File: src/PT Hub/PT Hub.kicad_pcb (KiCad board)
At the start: 2 copper layers, 18 parts, among them P1 20021511-00026T4LF, P2 39299043, P3 39299043, P4 39299043, P5 39299043, P6 39299043, P7 39299043, P8 39299043, P9 39299043

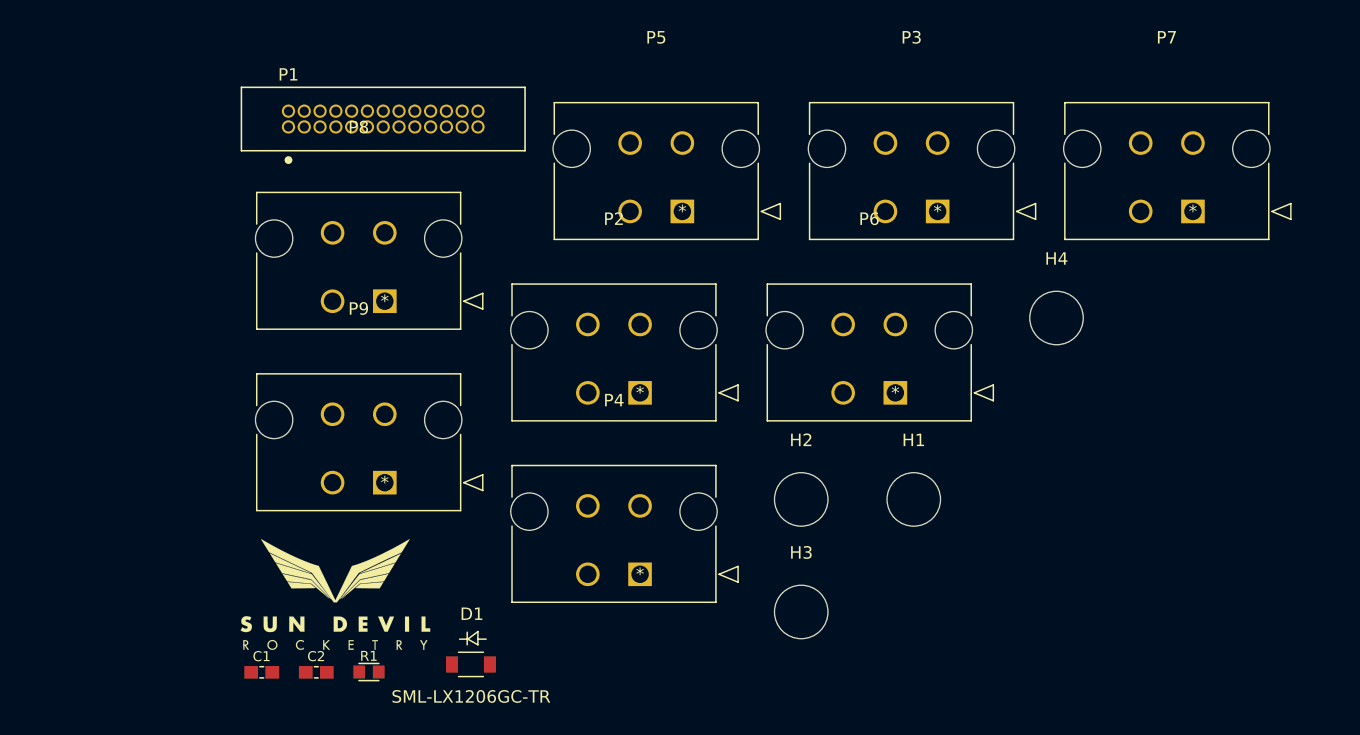
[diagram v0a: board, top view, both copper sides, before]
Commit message: most recent PCB changes as of 7/1
PT Hub PCB changes
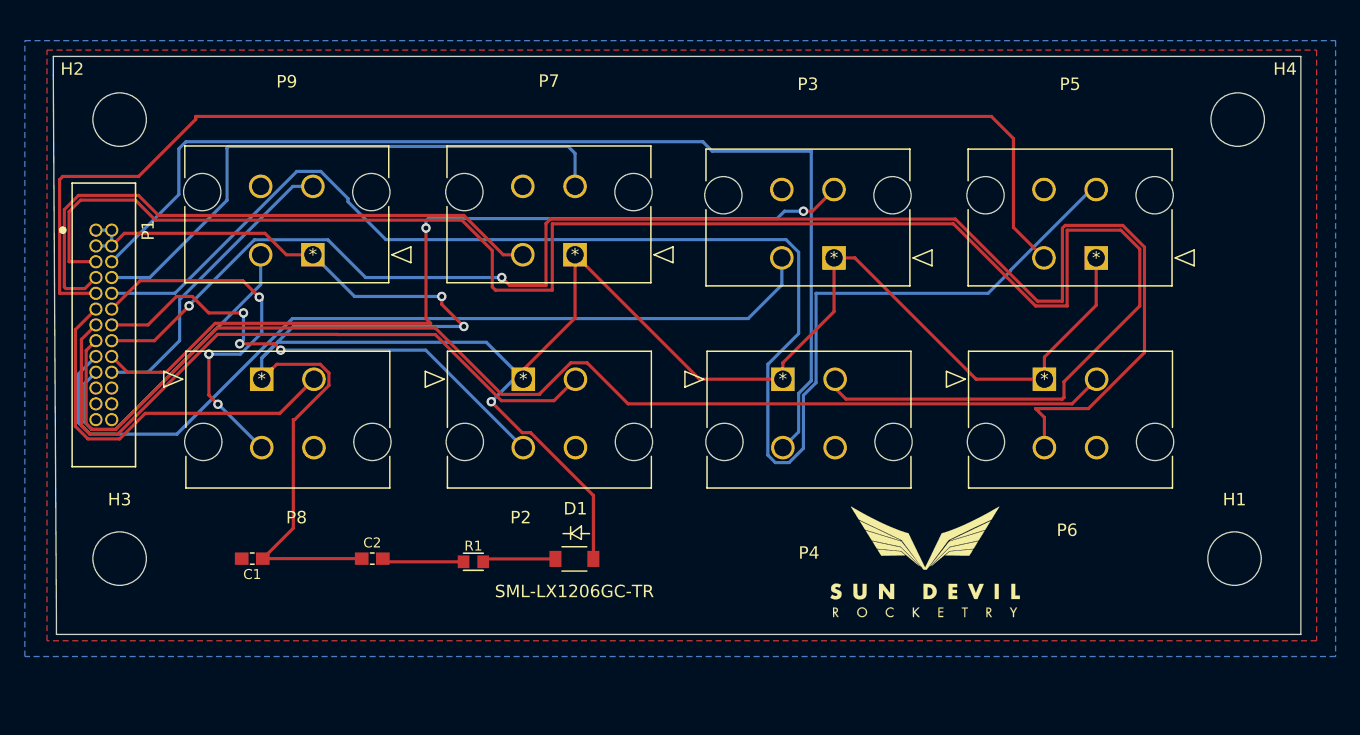
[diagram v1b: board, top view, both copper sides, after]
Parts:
- LOGO1: value Logo -> LOGO
- P2, P3, P4, P5, P6, P7, P8, P9: value 39299043 -> CON_39299043
- moved H2 62.8 mm to (76.2, 101.6)
- moved H3 55.0 mm to (76.2, 136.9)
- moved P7 49.8 mm to (112.8, 112.5)
- moved LOGO1 47.5 mm to (141.0, 136.9)
- moved P5 33.5 mm to (154.7, 112.7)
- moved P1 27.9 mm to (74.9, 118.1), turned to -90 degrees
- moved H1 26.2 mm to (165.9, 136.9)
- moved H4 21.6 mm to (166.1, 101.6)
- moved P4 19.4 mm to (129.5, 122.5), turned to 180 degrees
- moved P9 19.2 mm to (91.7, 112.5)
- moved R1 12.2 mm to (104.6, 137.2)
- moved P6 12.0 mm to (150.6, 122.5), turned to 180 degrees
- moved D1 11.9 mm to (112.8, 136.9)
- moved P8 11.7 mm to (87.6, 122.5), turned to 180 degrees
- moved C2 10.2 mm to (96.5, 136.9)
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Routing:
- net 5V: track 0.00 -> 205.4 mm, vias 0 -> 3
- net PT1+: track 0.00 -> 146.2 mm
- net PT6-: track 0.00 -> 125.1 mm, vias 0 -> 2
- net PT3-: track 0.00 -> 122.0 mm
- net PT3+: track 0.00 -> 102.4 mm
- net PT6+: track 0.00 -> 97.3 mm
- net PT1-: track 0.00 -> 87.5 mm
- net PT7-: track 0.00 -> 70.1 mm, vias 0 -> 2
- net PT7+: track 0.00 -> 70.0 mm
- net PT5+: track 0.00 -> 54.9 mm
- net PT2+: track 0.00 -> 48.5 mm
- net PT2-: track 0.00 -> 47.0 mm
- net PT5-: track 0.00 -> 41.0 mm, vias 0 -> 3
- net PT4+: track 0.00 -> 31.7 mm
- net PT4-: track 0.00 -> 30.6 mm, vias 0 -> 3
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- added copper zone on B.Cu, net Earth
- added copper zone on F.Cu, net Earth
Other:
- board outline added: 100.3 x 46.5 mm
